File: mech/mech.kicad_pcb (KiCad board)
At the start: 2 copper layers, 39 parts, among them P1 Pump_Motor_DC, P2 Pump_Motor_DC, T1 DS18B20, T2 DS18B20, U1 DHT22, U2 PCA9685PW

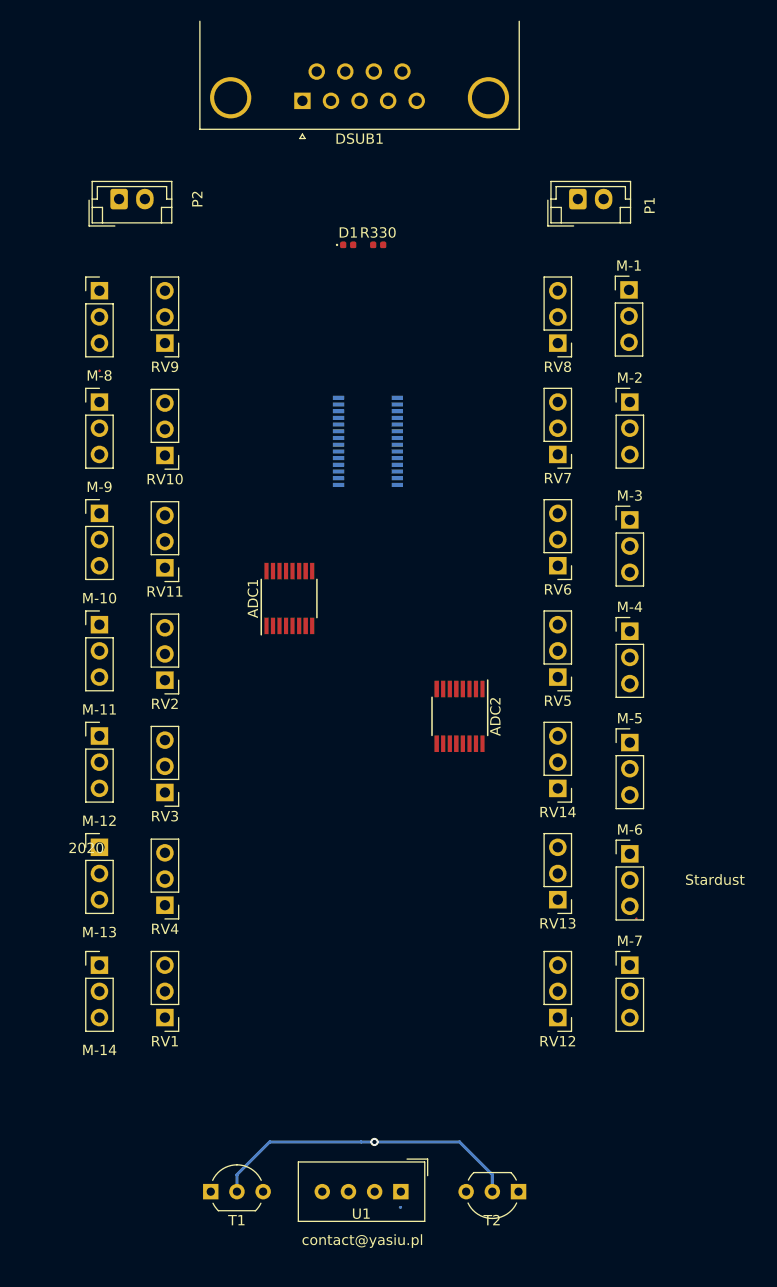
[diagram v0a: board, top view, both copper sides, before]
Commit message: final
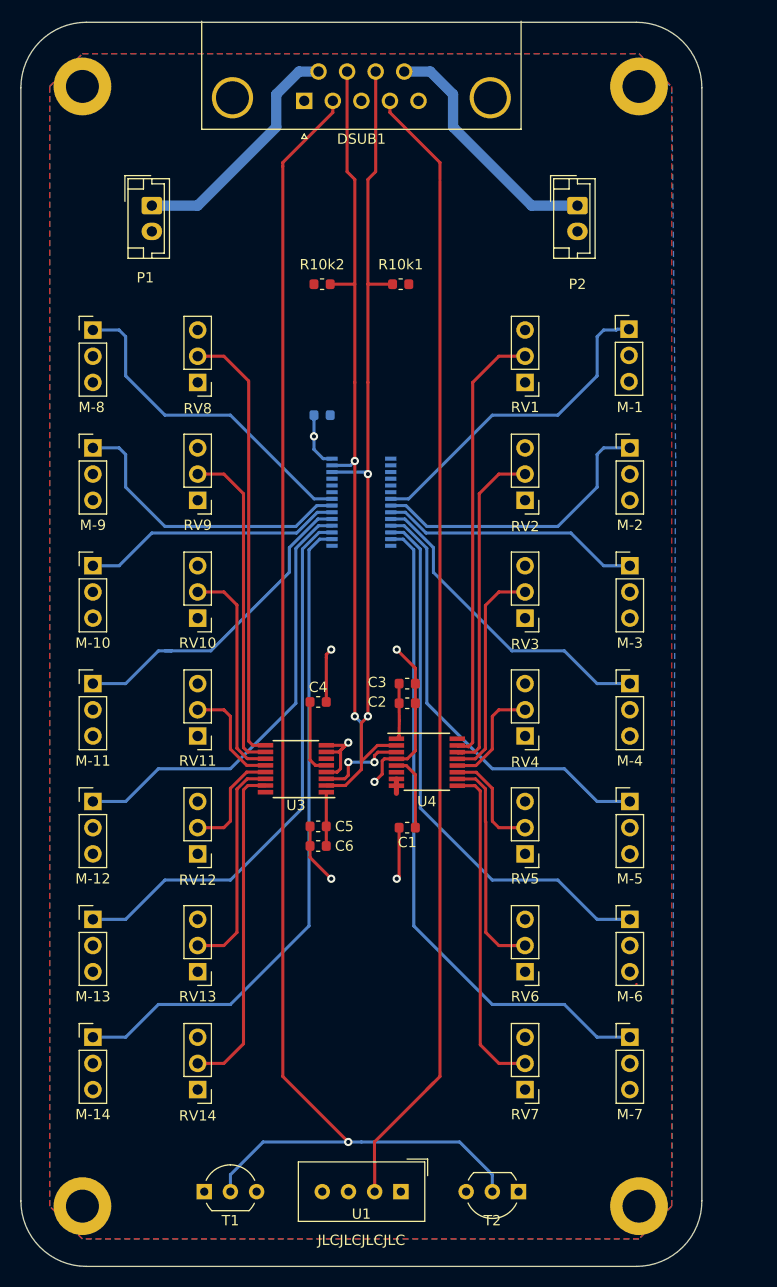
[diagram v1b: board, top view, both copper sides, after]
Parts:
- removed ADC1, ADC2: MAX11615, Package_SO:QSOP-16_3.9x4.9mm_P0.635mm
- removed D1: LED, LED_SMD:LED_0402_1005Metric
- removed R330: R, Resistor_SMD:R_0402_1005Metric
- removed the RV12 at (120.7, 191.8)
- removed the RV13 at (120.7, 180.3)
- removed the RV14 at (120.7, 169.5)
- removed the RV8 at (120.7, 126.4)
- added  : MountingHole_3.2mm_M3_DIN965_Pad, MountingHole:MountingHole_3.2mm_M3_DIN965_Pad, F.Cu at (74.5, 101.5)
- added  : MountingHole_3.2mm_M3_DIN965_Pad, MountingHole:MountingHole_3.2mm_M3_DIN965_Pad, F.Cu at (74.5, 210.1)
- added  : MountingHole_3.2mm_M3_DIN965_Pad, MountingHole:MountingHole_3.2mm_M3_DIN965_Pad, F.Cu at (128.5, 210.1)
- added  : MountingHole_3.2mm_M3_DIN965_Pad, MountingHole:MountingHole_3.2mm_M3_DIN965_Pad, F.Cu at (128.5, 101.5)
- added C0: C100nF, Resistor_SMD:R_0603_1608Metric, B.Cu at (97.8, 133.3)
- added C1: C100nF, Resistor_SMD:R_0603_1608Metric, F.Cu at (106.0, 173.4)
- added C2: 10nF, Resistor_SMD:R_0603_1608Metric, F.Cu at (106.0, 161.3)
- added C3: 100nF, Resistor_SMD:R_0603_1608Metric, F.Cu at (106.0, 159.4)
- added C4: C100nF, Resistor_SMD:R_0603_1608Metric, F.Cu at (97.4, 161.2)
- added C5: C10nF, Resistor_SMD:R_0603_1608Metric, F.Cu at (97.4, 173.2)
- added C6: C100nF, Resistor_SMD:R_0603_1608Metric, F.Cu at (97.4, 175.1)
- added R10k1: R, Resistor_SMD:R_0603_1608Metric, F.Cu at (105.4, 120.7)
- added R10k2: R, Resistor_SMD:R_0603_1608Metric, F.Cu at (97.8, 120.7)
- added RV1: R_POT, Connector_PinHeader_2.54mm:PinHeader_1x03_P2.54mm_Vertical, F.Cu at (117.5, 130.2)
- added RV2: R_POT, Connector_PinHeader_2.54mm:PinHeader_1x03_P2.54mm_Vertical, F.Cu at (117.5, 141.6)
- added RV3: R_POT, Connector_PinHeader_2.54mm:PinHeader_1x03_P2.54mm_Vertical, F.Cu at (117.5, 153.0)
- added RV4: R_POT, Connector_PinHeader_2.54mm:PinHeader_1x03_P2.54mm_Vertical, F.Cu at (117.5, 164.5)
- added U3: ADC128D818, Package_SO:TSSOP-16_4.4x5mm_P0.65mm, F.Cu at (95.2, 167.6)
- added U4: ADC128D818, Package_SO:TSSOP-16_4.4x5mm_P0.65mm, F.Cu at (108.0, 167.0)
- moved RV7 61.7 mm to (117.5, 198.8)
- moved P2 44.5 mm to (122.6, 113.0), turned to 270 degrees
- moved P1 41.3 mm to (81.3, 113.0), turned to 270 degrees
- moved RV14 39.8 mm to (85.7, 198.8)
- moved RV6 39.5 mm to (117.5, 187.3)
- moved RV11 27.5 mm to (85.7, 164.5)
- moved RV10 26.9 mm to (85.7, 153.0)
- moved RV8 18.3 mm to (85.7, 130.2)
- moved RV13 17.7 mm to (85.7, 187.3)
- moved RV5 17.4 mm to (117.5, 175.9)
- moved M-13 7.01 mm to (75.6, 182.2)
- moved M-14 7.01 mm to (75.6, 193.7)
- moved M-7 6.99 mm to (127.6, 193.7)
- moved M-12 6.38 mm to (75.6, 170.8)
- moved M-6 6.35 mm to (127.6, 182.2)
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- renumbered RV9 to RV10, RV1 to RV11, RV4 to RV12, RV3 to RV13, RV2 to RV14, RV11 to RV8, RV10 to RV9
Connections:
- DSUB1 pad 0: Net-(DSUB1-Pad0) -> GND
- DSUB1 pad 2: Pump-1 -> 1Wire
- DSUB1 pad 3: I2C-SDA -> (no net)
- DSUB1 pad 4: 1Wire -> DHT22
- DSUB1 pad 7: I2C-SCL -> I2C-SDA
- DSUB1 pad 8: DHT22 -> I2C-SCL
- DSUB1 pad 9: (no net) -> Pump-1
- U2 pad 1: (no net) -> GND
- U2 pad 14: (no net) -> GND
- U2 pad 2: (no net) -> GND
- U2 pad 23: (no net) -> GND
- U2 pad 24: (no net) -> GND
- U2 pad 3: (no net) -> GND
- U2 pad 4: (no net) -> GND
- U2 pad 5: (no net) -> GND
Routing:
- net DHT22: track 0.00 -> 111.2 mm
- net 1Wire: track 30.7 -> 136.9 mm
- net I2C-SCL: track 0.00 -> 82.3 mm, vias 0 -> 2
- net I2C-SDA: track 0.00 -> 81.3 mm, vias 0 -> 4
- net Net-(M-7-Pad1): track 0.00 -> 64.6 mm
- net Net-(M-14-Pad1): track 0.00 -> 64.6 mm
- net Net-(M-6-Pad1): track 0.00 -> 53.4 mm
- net Net-(M-13-Pad1): track 0.00 -> 53.4 mm
- net Net-(M-5-Pad1): track 0.00 -> 43.1 mm
- net Net-(M-12-Pad1): track 0.00 -> 43.1 mm
- net Net-(RV1-Pad2): track 0.00 -> 42.8 mm
- net Net-(RV8-Pad2): track 0.00 -> 42.7 mm
- net GND: track 0.02 -> 42.0 mm, vias 0 -> 6
- net Net-(RV2-Pad2): track 0.00 -> 32.2 mm
- net Net-(M-8-Pad1): track 0.00 -> 32.2 mm
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- added copper zone on F.Cu, net +5V
- added copper zone on B.Cu, net GND
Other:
- board outline added: 66 x 120.7 mm
- board text added: "Stardust 2020"
- board text removed: "2020"
- board text removed: "Stardust"
